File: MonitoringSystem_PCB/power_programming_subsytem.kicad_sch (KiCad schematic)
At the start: 17 parts, among them J2 UJ2-BH-W1-TH, Q1 SS8050-G, Q2 SS8050-G, U1 CP2102N-Axx-xQFN28, U6 LM1117MP-3.3

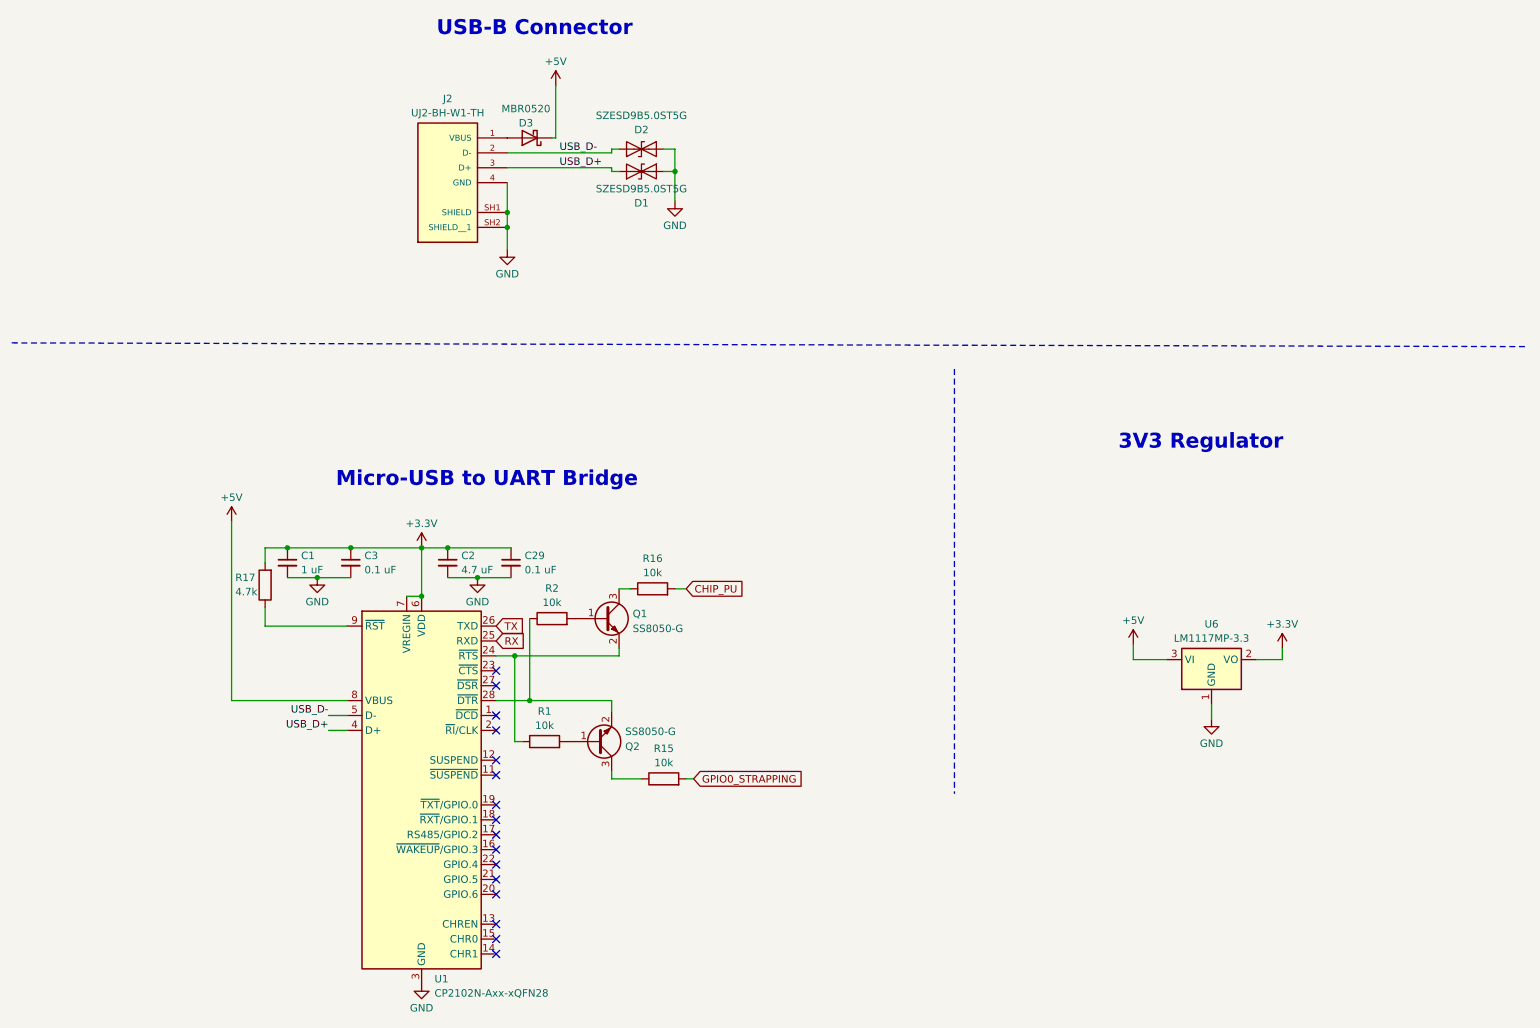
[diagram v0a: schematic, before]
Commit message: most recent pcb
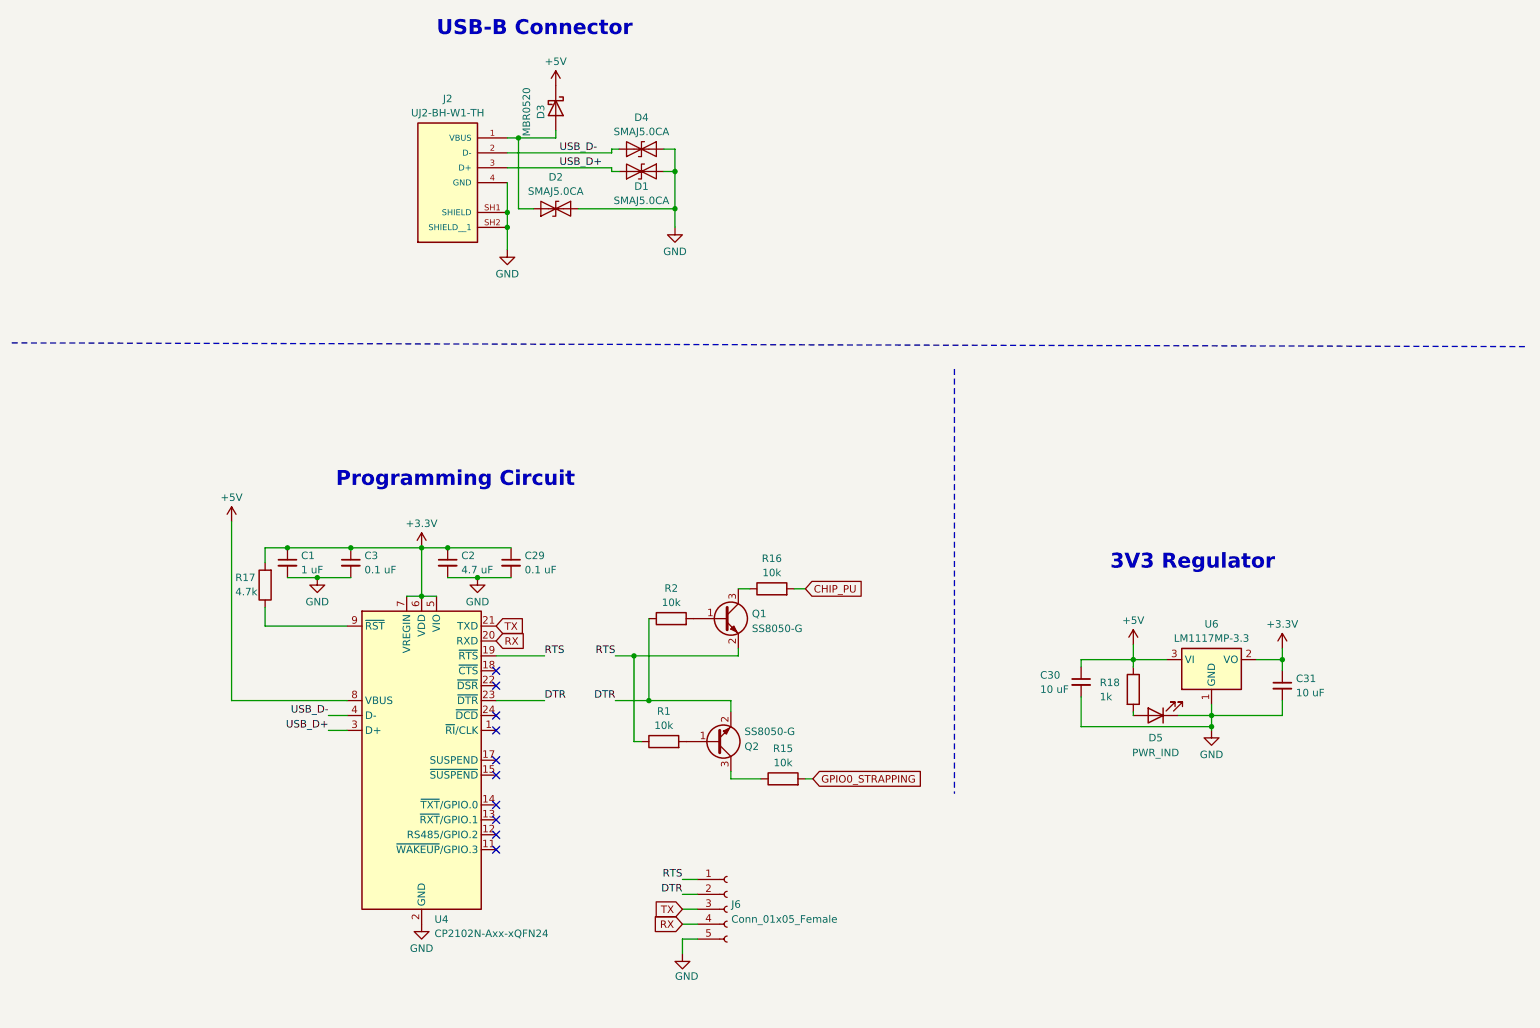
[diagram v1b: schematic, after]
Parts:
- removed D1, D2: SZESD9B5.0ST5G, Diode_SMD:D_SOD-923, symbol Diode:SZESD9B5.0ST5G
- removed U1: CP2102N-Axx-xQFN28, Package_DFN_QFN:QFN-28-1EP_5x5mm_P0.5mm_EP3.35x3.35mm, symbol Interface_USB:CP2102N-Axx-xQFN28
- added C30, C31: 10 uF, Capacitor_SMD:C_0805_2012Metric, symbol Device:C_Small
- added D1, D2, D4: SMAJ5.0CA, Diode_SMD:D_SMA, symbol Diode:SMAJ5.0CA
- added D5: PWR_IND, LED_SMD:LED_0805_2012Metric, symbol Device:LED
- added J6: Conn_01x05_Female, Connector_PinHeader_2.54mm:PinHeader_1x05_P2.54mm_Vertical, symbol Connector:Conn_01x05_Female
- added R18: 1k, Resistor_SMD:R_0805_2012Metric, symbol Device:R
- added U4: CP2102N-Axx-xQFN24, Package_DFN_QFN:QFN-24-1EP_4x4mm_P0.5mm_EP2.6x2.6mm, symbol Interface_USB:CP2102N-Axx-xQFN24
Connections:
- net +3.3V: now also C31.1, U4.5 (VIO), U4.6 (VDD), U4.7 (VREGIN)
- net +5V: now also C30.1, R18.1, U4.8 (VBUS)
- net GND: now also C30.2, C31.2, D1.2 (A2), D2.2 (A2), D4.2 (A2), D5.1 (K), J6.5 (Pin_5), U4.2 (GND), U4.25 (GND)
- net RX: now also J6.4 (Pin_4), U4.20 (RXD)
- net TX: now also J6.3 (Pin_3), U4.21 (TXD)
- net USB_D+: now also D1.1 (A1), U4.3 (D+)
- net USB_D-: now also D4.1 (A1), U4.4 (D-)
- net DTR: now reaches Q2.2 (E), R2.1
- net DTR: now also J6.2 (Pin_2), U4.23 (~{DTR})
- net at R17.1: now also U4.9 (~{RST})
- net RTS: now reaches Q1.2 (E), R1.1
- net RTS: now also J6.1 (Pin_1), U4.19 (~{RTS})
- net at D3.2 (A), J2.1 (VBUS): now also D2.1 (A1)
- new net: D5.2 (A), R18.2
- no-connect marks 16 -> 10
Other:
- note added: "Programming Circuit"
- note removed: "Micro-USB to UART Bridge"
- moved on the sheet: D3, Q1, Q2, R1, R15, R16, R2
